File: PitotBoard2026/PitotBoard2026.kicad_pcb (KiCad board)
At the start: 2 copper layers, 60 x 41.9 mm, 74 parts, among them J1 RJ25, J2 ICSP(, J3 Conn_01x04_Socket, J4 Conn_01x04_Pin, J5 Conn_01x04_Socket, J6 Conn_01x04_Pin, SW1 RST, U1 ATmega328PB-A, U10 MCP25625-x-SS, U11 FXMA2102, U2 M78AR05-0.5, U3 SDP32, U4 SLIP, U5 TPS76133SF5, U7 SLIP, U9 BME280, Y1 16MHz, Y3 16MHz

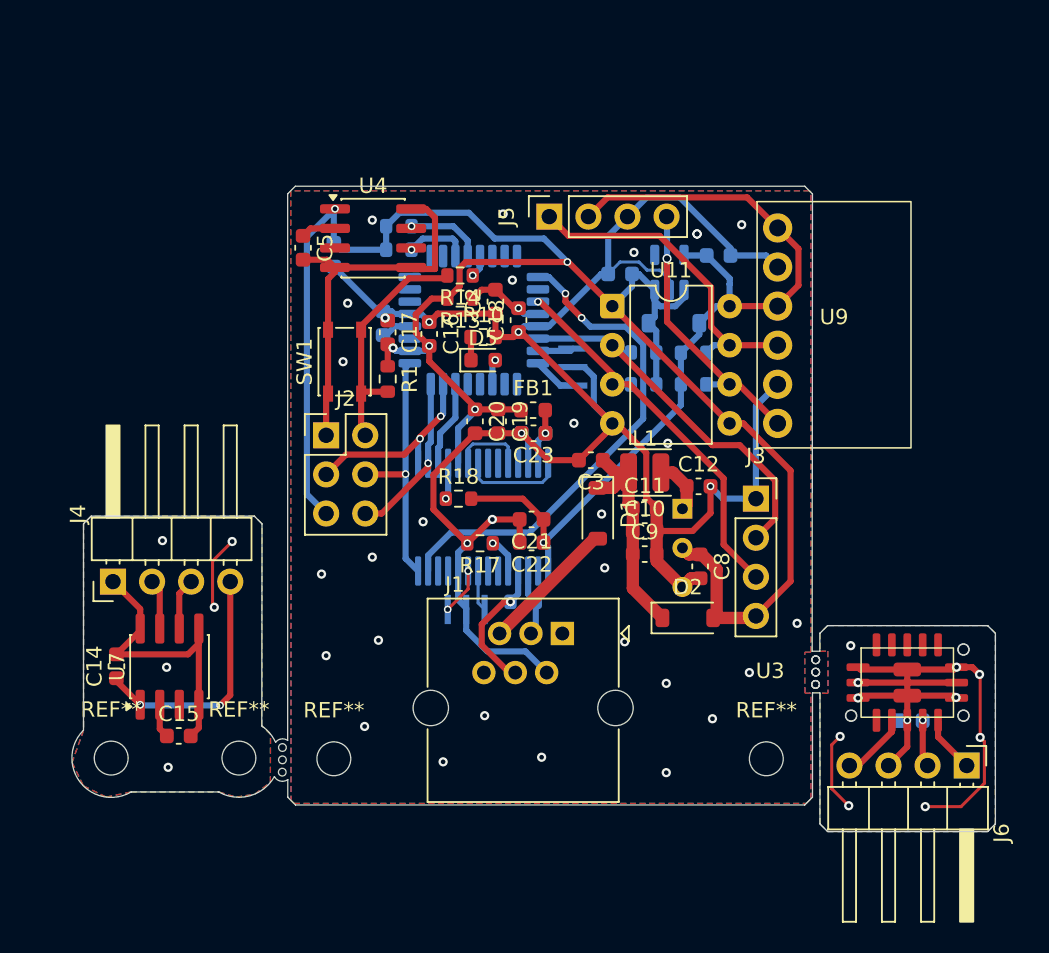
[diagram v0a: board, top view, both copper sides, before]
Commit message: Add files via upload
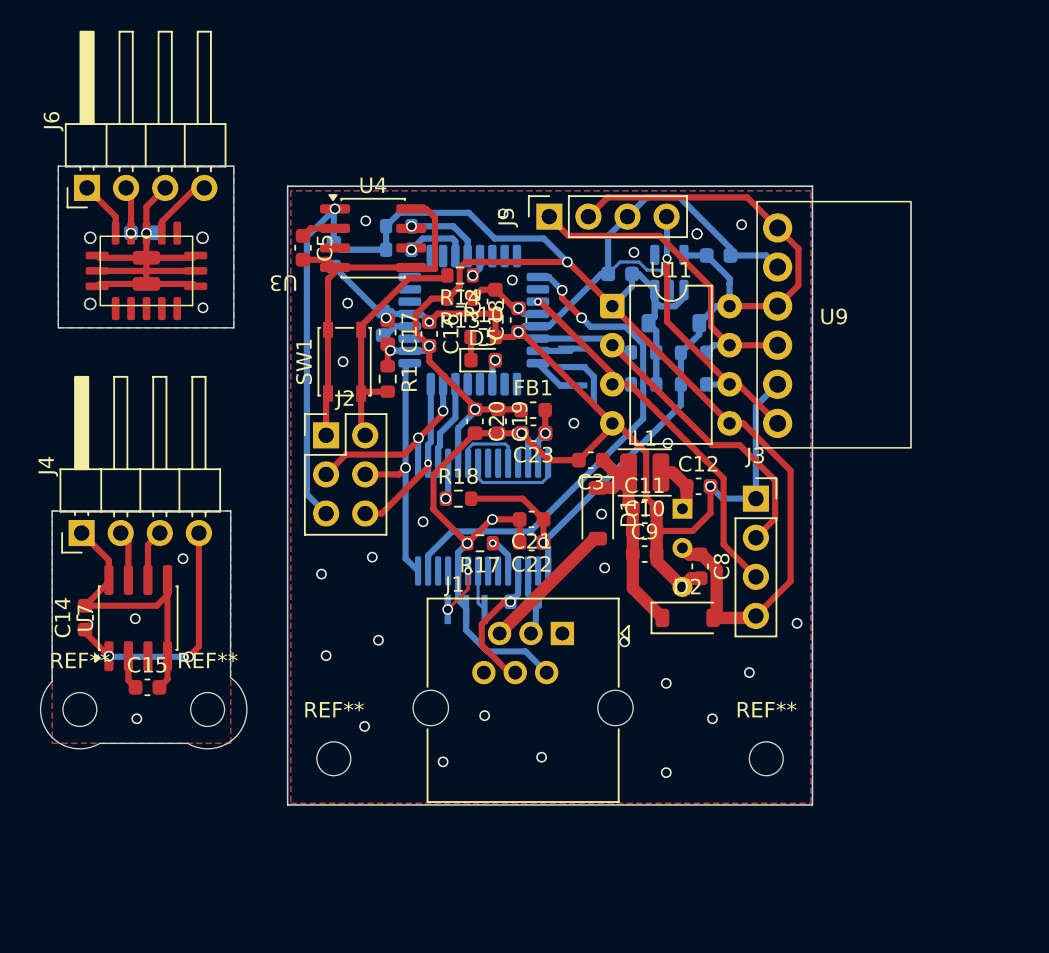
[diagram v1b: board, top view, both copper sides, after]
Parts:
- removed ? (x7): , 
- removed the REF** at (180.5, 141.6)
- removed the REF** at (145.8, 147.3)
- moved J6 68.4 mm to (133.2, 109.3), turned to 90 degrees
- moved C27 59.1 mm to (136.8, 112.2), turned to 0 degrees
- moved U3 56.2 mm to (137.0, 114.7), turned to 180 degrees
- moved REF** 3.75 mm to (132.7, 143.2)
- moved C15 3.75 mm to (137.1, 141.8)
- moved REF** 3.75 mm to (141.0, 143.2)
- moved U7 3.75 mm to (136.5, 137.3)
- moved C14 3.75 mm to (133.0, 137.2)
- moved J4 3.75 mm to (132.8, 131.7)
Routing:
- net GND2: track 45.4 -> 26.9 mm, vias 11 -> 2
- net GND1: track 24.8 -> 19.9 mm, vias 5 -> 3
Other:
- board size 60 x 41.9 mm -> 50.2 x 41.5 mm
